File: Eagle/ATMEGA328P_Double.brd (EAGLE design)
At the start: 150 x 100 mm, 89 parts, among them CN1 SEG_1, CN2 SEG_2, CN3 SEG_3, CN4 To I2C Device, CN6 SW1, CN7 SW2, CN8 SW3, CN9 1PPS, IC1 74HC595, IC2 74HC595, IC4 TBD62083, IC5 TBD62083, IC7 74HC595, IC8 TBD62083

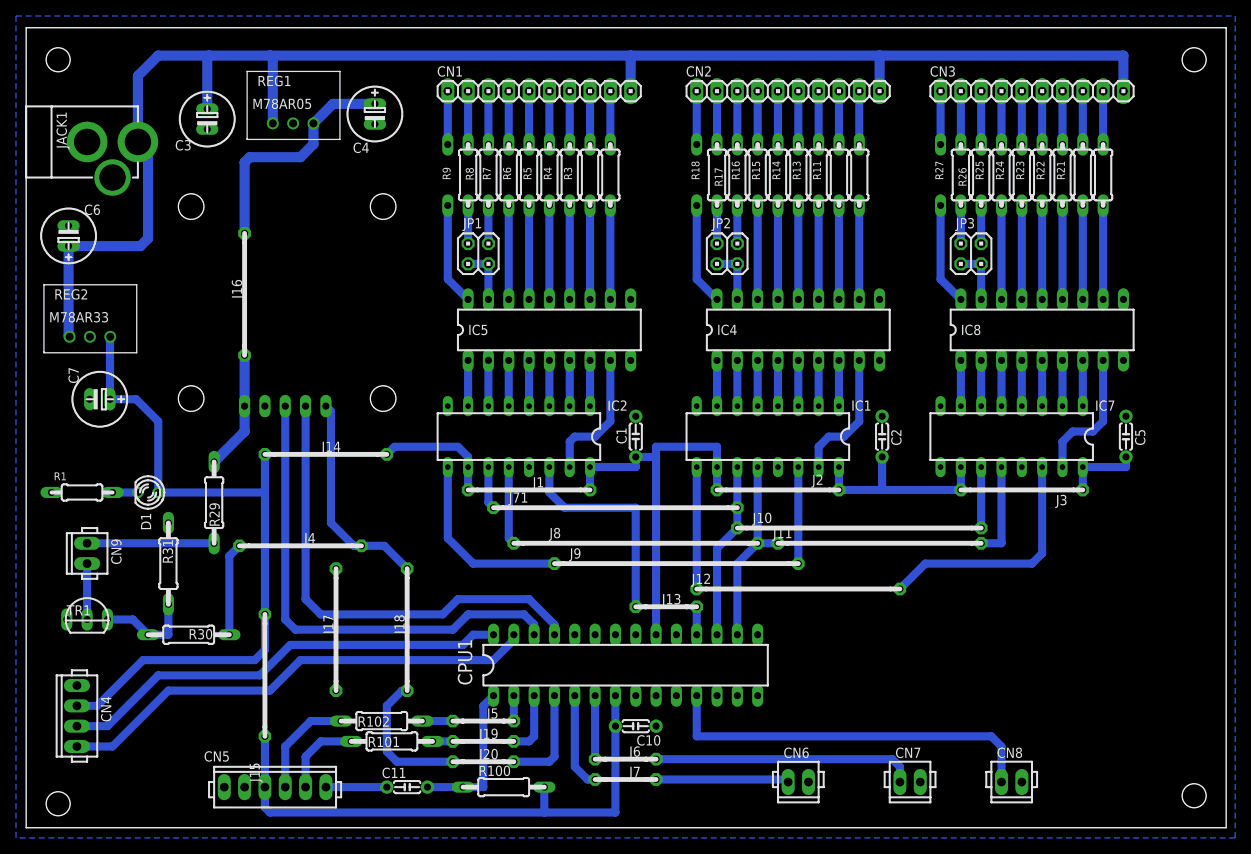
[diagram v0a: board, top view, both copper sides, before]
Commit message: Eagle FIle UPload
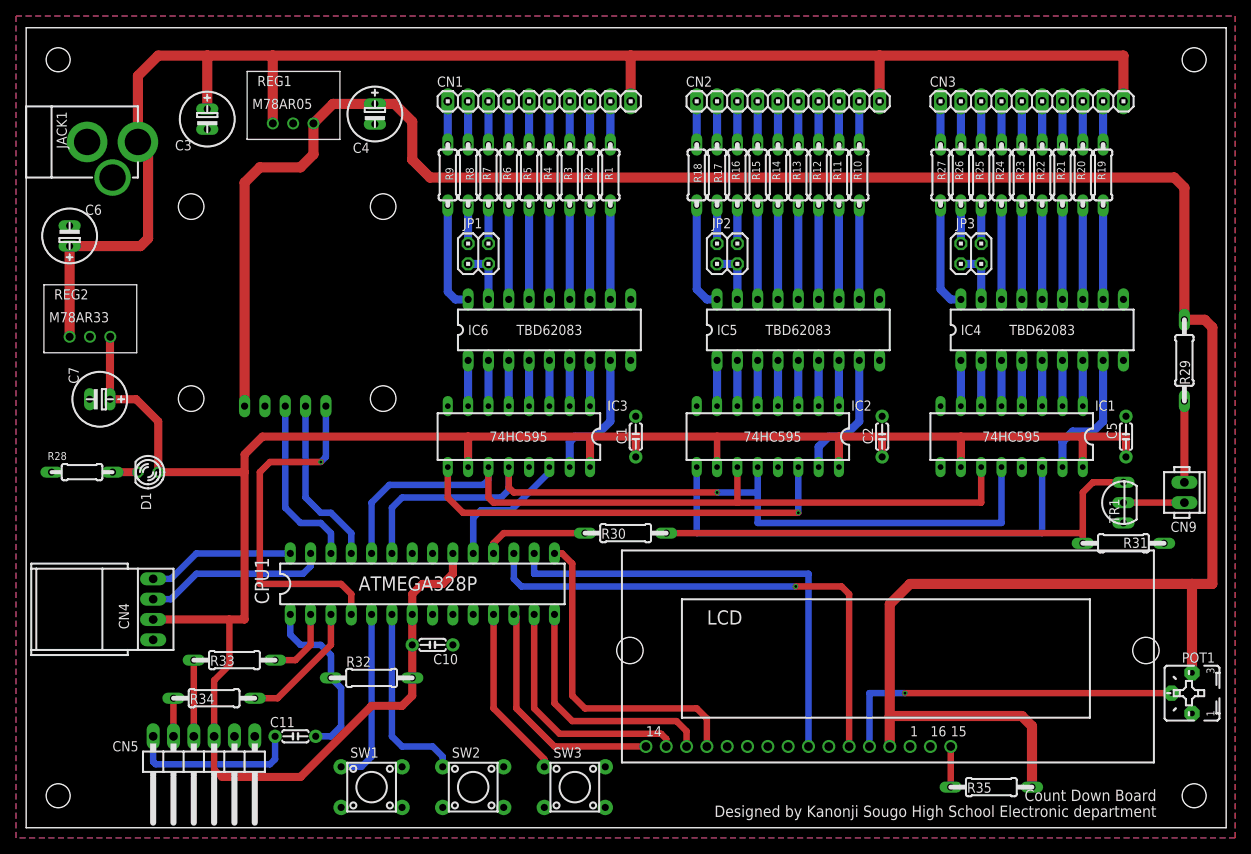
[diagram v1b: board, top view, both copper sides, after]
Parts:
- removed CN6: SW1, 1-conn-jst:2P-S
- removed CN7: SW2, 1-conn-jst:2P-S
- removed CN8: SW3, 1-conn-jst:2P-S
- removed IC7: 74HC595, MyLib:DIL16
- removed IC8: TBD62083, microchip:DIL18
- removed J1, J14, J15, J16, J17, J18, J2, J3, J4: (no value), 1-jumper:15
- removed J10, J71, J8, J9: (no value), 1-jumper:30
- removed J11, J12: (no value), 1-jumper:25
- removed J13, J19, J20, J5, J6, J7: (no value), 1-jumper:07
- removed R100: 10k, akihabara:0207/10
- removed R101, R102: 1k, akihabara:0207/10
- added IC3: 74HC595, MyLib:DIL16
- added IC6: TBD62083, microchip:DIL18
- added LCD: (no value), 1-display:SD1602H
- added POT1: (no value), MyLib:POT_B25P
- added R32: 10k, akihabara:0207/10
- added R33, R34: 1k, akihabara:0207/10
- added R35: 150, akihabara:0207/10
- added SW1, SW2, SW3: (no value), 1-sw:B3F-10XX
- CN4: device 1-conn-jst:4P-S -> 1-conn-jst:4P-L
- CN5: value (none) -> Writer; device 1-conn-jst:6P-S -> pinhead:1X06/90
- R1: device akihabara:0204/7 -> akihabara:0207/7
- R10, R12, R19, R2, R20: value 430 -> 1k
- R28: value 430 -> 1k; device akihabara:0207/7 -> akihabara:0204/7
- moved CN9 137.4 mm to (144.8, 41.9), turned to 90 degrees
- moved R28 132.9 mm to (6.99, 44.5), turned to 180 degrees
- moved TR1 130.4 mm to (137.2, 40.6), turned to 90 degrees
- moved R29 122.6 mm to (144.8, 58.4)
- moved R31 119.4 mm to (137.2, 35.6), turned to 180 degrees
- moved R1 77.0 mm to (73.0, 81.6), turned to 90 degrees
- moved R30 56.1 mm to (74.9, 36.8), turned to 0 degrees
- moved IC2 31.1 mm to (92.7, 48.9)
- moved IC5 31.1 mm to (96.5, 62.2)
- moved IC1 30.5 mm to (123.2, 48.9)
- moved IC4 30.5 mm to (127.0, 62.2)
- moved R19 30.5 mm to (134.6, 81.6)
- moved C10 27.4 mm to (50.8, 22.9)
- moved CPU1 27.4 mm to (49.5, 30.5)
- moved R12 26.0 mm to (99.1, 81.6)
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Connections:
- net COM_SEG1_IN renamed IN_SEG3_A
- net COM_SEG2_IN renamed IN_SEG3_G
- net COM_SEG3_IN renamed IN_SEG3_F
- net IN_SEG_A renamed IN_SEG2_D
- net IN_SEG_B renamed IN_SEG2_C
- net IN_SEG_C renamed IN_SEG2_E
- net IN_SEG_D renamed IN_SEG2_A
- net IN_SEG_DP renamed IN_SEG2_F
- net IN_SEG_E renamed IN_SEG2_G
- net IN_SEG_F renamed IN_SEG2_B
- net IN_SEG_G renamed IN_SEG2_DP
- net SEG_F_IN renamed IN_SEG3_B
- net TR2_IN renamed IN_SEG3_E
- net TR3_IN renamed IN_SEG3_D
- net TR5_IN renamed IN_SEG3_C
- net TR４_IN renamed IN_SEG3_DP
- removed net 1PPS: CPU1.4, GPS1.1PPS, J18.1, J18.2, J20.1, J20.2, J4.1, J4.2, R30.1
- removed net COM_SEG1_IN1: IC7.2, IC8.6
- removed net COM_SEG2_IN1: IC7.1, IC8.7
- removed net COM_SEG3_IN1: IC7.15, IC8.8
- removed net CTS: C11.1, CN5.1
- removed net RXD<-TXD: CN5.2, R101.1
- removed net S$1: CPU1.23
- removed net SEG_F_IN1: IC7.3, IC8.5
- removed net SW1/D2: CN6.1, CPU1.5, J7.1, J7.2
- removed net SW2/D3: CN7.1, CPU1.6, J6.1, J6.2
- removed net SW4: CPU1.14
- removed net TR2_IN1: IC7.4, IC8.4
- removed net TR3_IN1: IC7.5, IC8.3
- removed net TR5_IN1: IC7.7, IC8.1
- removed net TR４_IN1: IC7.6, IC8.2
- new net 1PPS/D2: CPU1.4, GPS1.1PPS
- new net DB4: CPU1.15, LCD.11
- new net DB5: CPU1.14, LCD.12
- new net DB6: CPU1.13, LCD.13
- new net DB7: CPU1.12, LCD.14
- new net DTR: C11.1, CN5.6
- new net EN: CPU1.16, LCD.6
- new net IN_SEG1_A: IC3.2, IC6.6
- new net IN_SEG1_B: IC3.3, IC6.5
- new net IN_SEG1_C: IC3.7, IC6.1
- new net IN_SEG1_D: IC3.5, IC6.3
- new net IN_SEG1_DP: IC3.6, IC6.2
- new net IN_SEG1_E: IC3.4, IC6.4
- new net IN_SEG1_F: IC3.15, IC6.8
- new net IN_SEG1_G: IC3.1, IC6.7
- new net LCD_ANODE: LCD.15, R35.1
- new net OUT_1PPS: CPU1.18, R30.1
- new net RS: CPU1.17, LCD.4
- new net RXI<-TXD: CN5.5, R34.1
- new net SW1: CPU1.5, SW1.1
- new net SW2: CPU1.6, SW2.1
- new net VO: LCD.3, POT1.S
- net +3.3V: now also CN5.3, IC3.10, IC3.16, R32.2; no longer CN5.4, IC7.10, IC7.16, J1.1, J1.2, J14.1, J14.2, J15.1, J15.2, J2.1, J2.2, J3.1, J3.2, R100.2
- net +5V: now also LCD.2, POT1.E, R35.2; no longer J16.1, J16.2
- net A4/SDA: now also CN4.3; no longer CN4.4
- net A5/SCL: now also CN4.4; no longer CN4.3
- net D1_A: now also R28.1; no longer R1.1
- net GND: now also C7.-, CN5.1, IC3.13, IC3.8, IC6.9, LCD.1, LCD.16, LCD.5, POT1.A, R28.2, SW1.4, SW2.4, SW3.4; no longer CN5.6, CN6.2, CN7.2, CN8.2, IC7.13, IC7.8, IC8.9, J17.1, J17.2, R1.2
- net OUT_LED_A: now also CN9.2; no longer CN9.1
- net OUT_LED_K: now also CN9.1; no longer CN9.2
- net OUT_SEG1_A: now also IC6.13; no longer IC5.13
- net OUT_SEG1_B: now also IC6.14; no longer IC5.14
- net OUT_SEG1_C: now also IC6.18, R9.2; no longer IC5.18, R9.1
- net OUT_SEG1_D: now also IC6.16; no longer IC5.16
- net OUT_SEG1_E: now also IC6.15; no longer IC5.15
- net OUT_SEG1_F: now also IC6.11, R1.1; no longer IC5.11, R12.1
- net OUT_SEG1_G: now also IC6.12; no longer IC5.12
- net OUT_SEG1__DP: now also IC6.17; no longer IC5.17
- net OUT_SEG2_A: now also IC5.13, R12.1; no longer IC4.13, R11.1
- net OUT_SEG2_B: now also IC5.14; no longer IC4.14
- net OUT_SEG2_C: now also IC5.18, R18.2; no longer IC4.18, R18.1
- net OUT_SEG2_D: now also IC5.16; no longer IC4.16
- net OUT_SEG2_DP: now also IC5.17; no longer IC4.17
- net OUT_SEG2_E: now also IC5.15; no longer IC4.15
- net OUT_SEG2_F: now also IC5.11, R10.1; no longer IC4.11, R19.1
- net OUT_SEG2_G: now also IC5.12, R11.1; no longer IC4.12, R10.1
- net OUT_SEG3_A: now also IC4.13; no longer IC8.13
- net OUT_SEG3_B: now also IC4.14; no longer IC8.14
- net OUT_SEG3_C: now also IC4.18, R27.2; no longer IC8.18, R27.1
- net OUT_SEG3_D: now also IC4.16; no longer IC8.16
- net OUT_SEG3_DP: now also IC4.17; no longer IC8.17
- net OUT_SEG3_E: now also IC4.15; no longer IC8.15
- net OUT_SEG3_F: now also IC4.11, R19.1; no longer IC8.11, R28.1
- net OUT_SEG3_G: now also IC4.12; no longer IC8.12
- net QH1->SER: now also IC2.14, IC3.9; no longer IC1.14, IC2.9, J9.1, J9.2
- net QH2-SER: now also IC1.14, IC2.9; no longer IC1.9, IC7.14, J12.1, J12.2
- net RCLK: now also CPU1.23, IC3.12; no longer CPU1.16, IC7.12, J11.1, J11.2, J8.1, J8.2
- net RST: now also R32.1; no longer R100.1
- net RXD: now also R33.2; no longer J5.1, J5.2, R102.2
- net SCLK: now also CPU1.24, IC3.11; no longer CPU1.17, IC7.11, J10.1, J10.2, J71.1, J71.2
- net SEG1_C: now also R9.1; no longer R9.2
- net SEG1_F: now also R1.2; no longer R12.2
- net SEG2_A: now also R12.2; no longer R11.2
- net SEG2_C: now also R18.1; no longer R18.2
- net SEG2_F: now also R10.2; no longer R19.2
- net SEG2_G: now also R11.2; no longer R10.2
- net SEG3_C: now also R27.1; no longer R27.2
- net SEG3_F: now also R19.2; no longer R28.2
- net SER/D12: now also CPU1.19, IC3.14; no longer CPU1.18, IC2.14, J13.1, J13.2
- net SW3/D4: now also SW3.1; no longer CN8.1
- net TXD: now also R34.2; no longer J19.1, J19.2, R101.2
- net TXD->RXD: now also CN5.4, R33.1; no longer CN5.3, R102.1
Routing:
- net +5V: track 44.6 -> 307.5 mm
- net 1PPS: track 69.2 -> 0.00 mm
- net RS: track 0.00 -> 64.9 mm, vias 0 -> 1
- net SCLK: track 35.0 -> 98.3 mm
- net EN: track 0.00 -> 58.4 mm
- net RCLK: track 46.4 -> 102.5 mm, vias 0 -> 1
- net TR1_B: track 12.2 -> 64.0 mm
- net VO: track 0.00 -> 44.5 mm, vias 0 -> 1
- net 1PPS/D2: track 0.00 -> 43.9 mm, vias 0 -> 1
- net DB4: track 0.00 -> 40.8 mm
- net SW2/D3: track 40.7 -> 0.00 mm
- net A5/SCL: track 57.4 -> 18.5 mm
- net GPS_TXD: track 60.9 -> 22.3 mm
- net GPS_RXD: track 59.4 -> 21.5 mm
- net A4/SDA: track 60.8 -> 23.0 mm
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- added copper zone on layer 1, net GND
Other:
- board text added: "Count Down Board Designed by Kanonji Sougo High School Electronic department"
